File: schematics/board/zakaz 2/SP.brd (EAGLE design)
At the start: 30 x 46 mm, 15 parts

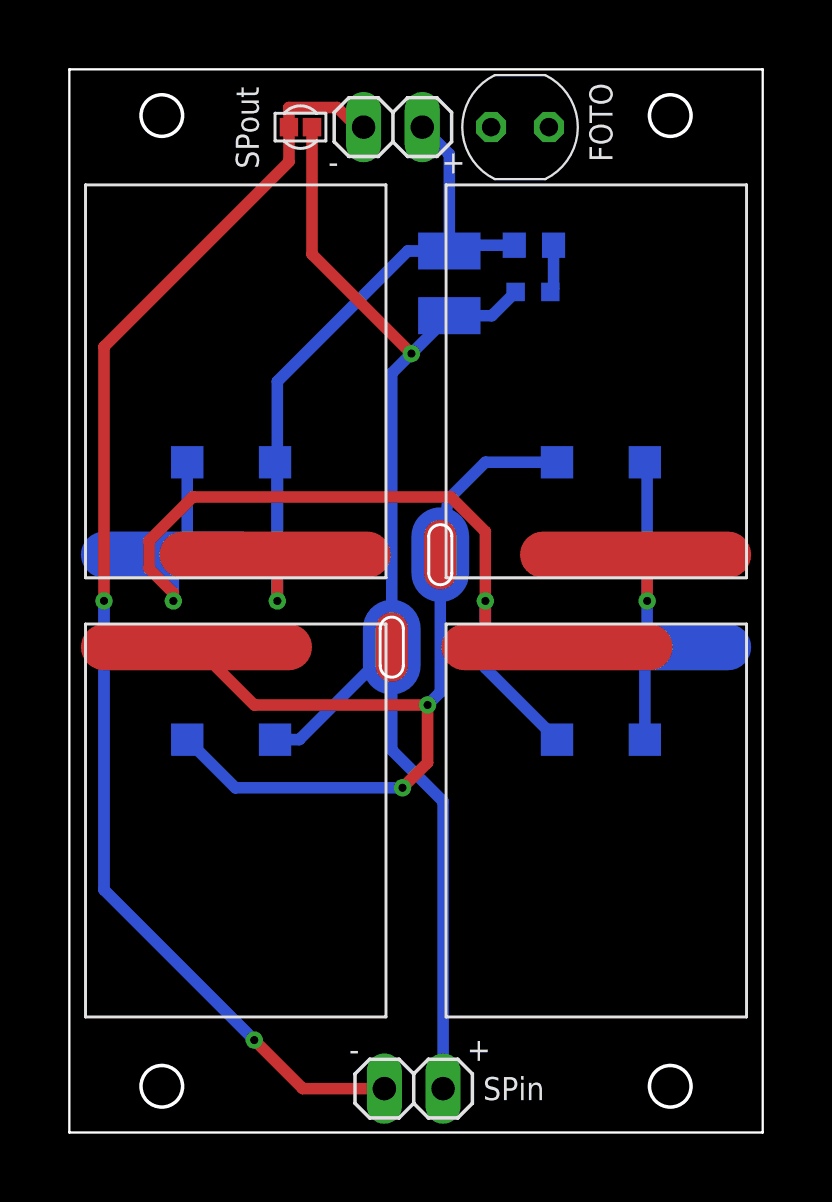
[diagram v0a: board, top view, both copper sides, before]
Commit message: Новые версии плат
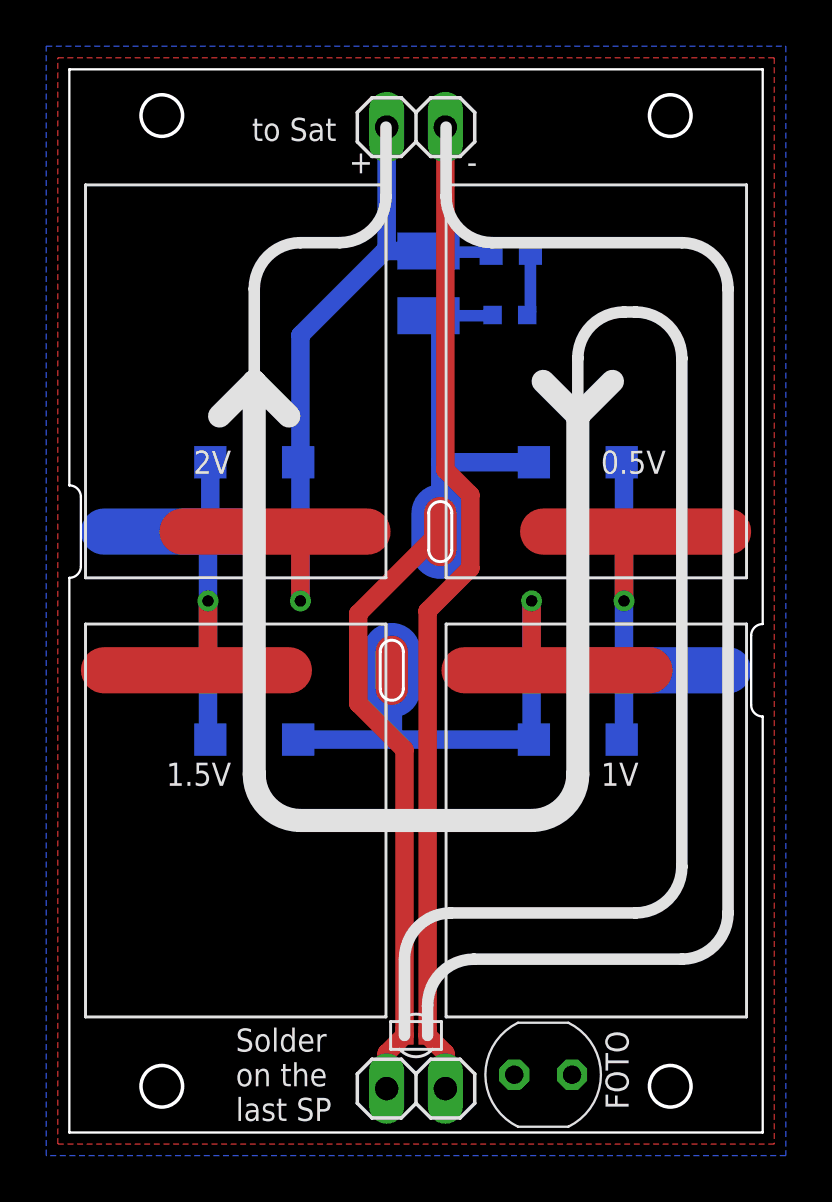
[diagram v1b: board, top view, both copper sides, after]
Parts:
- U$2: value SOLAR-2_1 -> SOLAR-2_0; device KNPN-2023:SOLAR_1-2 -> KNPN-2023:SOLAR_0-2
- U$3: value SOLAR-2_0 -> SOLAR-2_1; device KNPN-2023:SOLAR_0-2 -> KNPN-2023:SOLAR_1-2
- moved FOTO 41.0 mm to (20.5, 2.50)
- moved U$7 39.6 mm to (15.0, 4.20), turned to 0 degrees
- moved U$4 24.6 mm to (22.8, 32.5), turned to 90 degrees
- moved D4 19.2 mm to (22.0, 29.0), turned to 180 degrees
- moved U$3 19.0 mm to (22.8, 13.5), turned to 270 degrees
- moved U$2 15.6 mm to (7.20, 13.5)
- moved D2 15.0 mm to (8.00, 17.0)
- moved D3 12.0 mm to (22.0, 17.0), turned to 0 degrees
- moved PWR 1.41 mm to (19.1, 35.4)
- moved R1 1.04 mm to (19.1, 38.1)
- moved D1 1.00 mm to (8.00, 29.0)
- moved JP1 1.00 mm to (15.0, 43.5), turned to 180 degrees
- moved C1 0.90 mm to (15.5, 36.7)
- moved SP-OUT 0.10 mm to (15.0, 1.90), turned to 0 degrees
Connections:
- net N$2: now also U$2.OUT-2, U$2.OUT-21; no longer U$2.OUT
- net N$3: now also U$3.OUT; no longer U$3.OUT-2, U$3.OUT-21
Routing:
- net N$1: track 40.6 -> 17.1 mm, vias 2 -> 1
- net N$3: track 39.9 -> 16.8 mm, vias 2 -> 1
- net SP+-: track 57.0 -> 43.5 mm, vias 1 -> 0
- net SP-: track 56.4 -> 43.1 mm, vias 2 -> 0
- net N$2: track 15.0 -> 23.3 mm
- net SP+: track 36.1 -> 30.8 mm
- net N$4: track 2.08 -> 2.78 mm
- added copper zone on layer 1, net SP-
- added copper zone on layer 16, net SP-
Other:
- outline, holes or cut-outs redrawn
- board text added: "0.5V"
- board text added: "1.5V"
- board text added: "1V"
- board text added: "2V"
- board text added: "Solder on the last SP"
- board text added: "to Sat"
- board text removed: "SPin"
- board text removed: "SPout"
